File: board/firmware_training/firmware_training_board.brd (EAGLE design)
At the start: 68.6 x 53.4 mm, 17 parts, among them J1 GY-521-MPU-6050, SW1 PTS645, SW2 PTS645

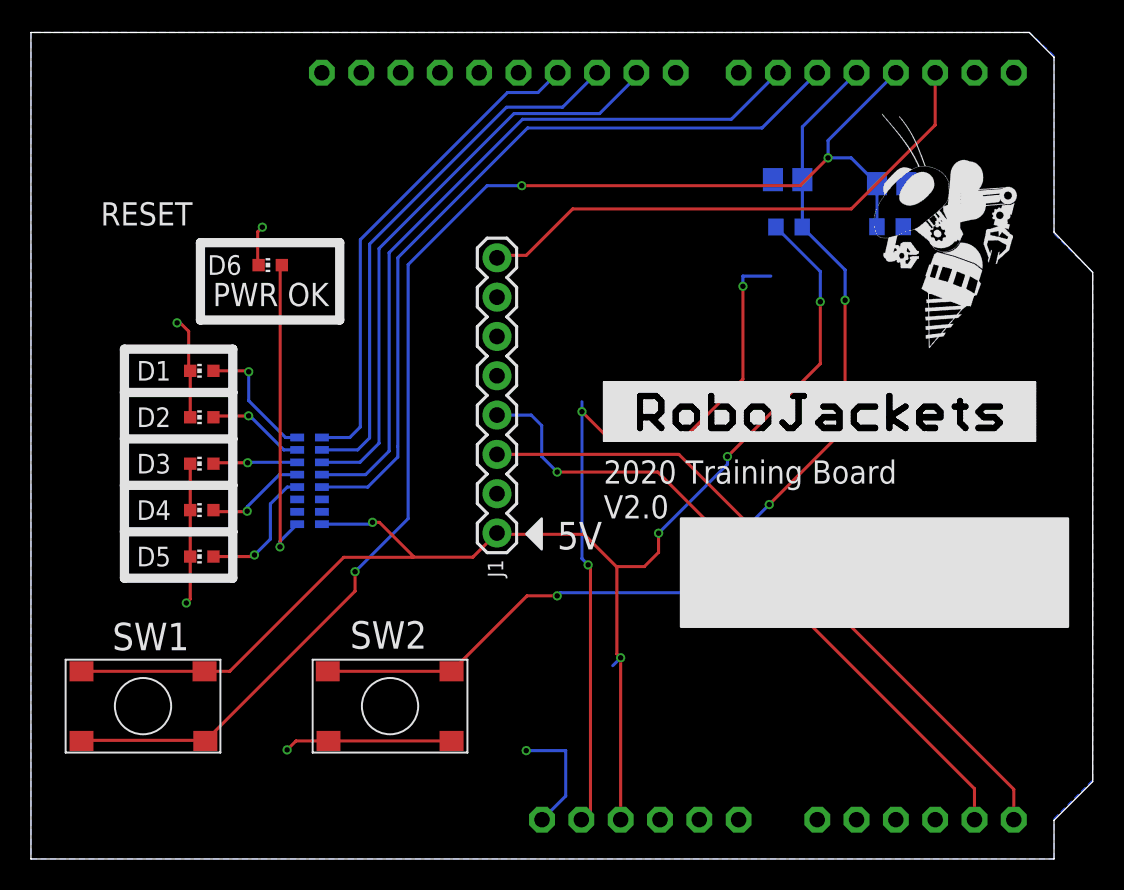
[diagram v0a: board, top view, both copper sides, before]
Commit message: Finished schematic, started board
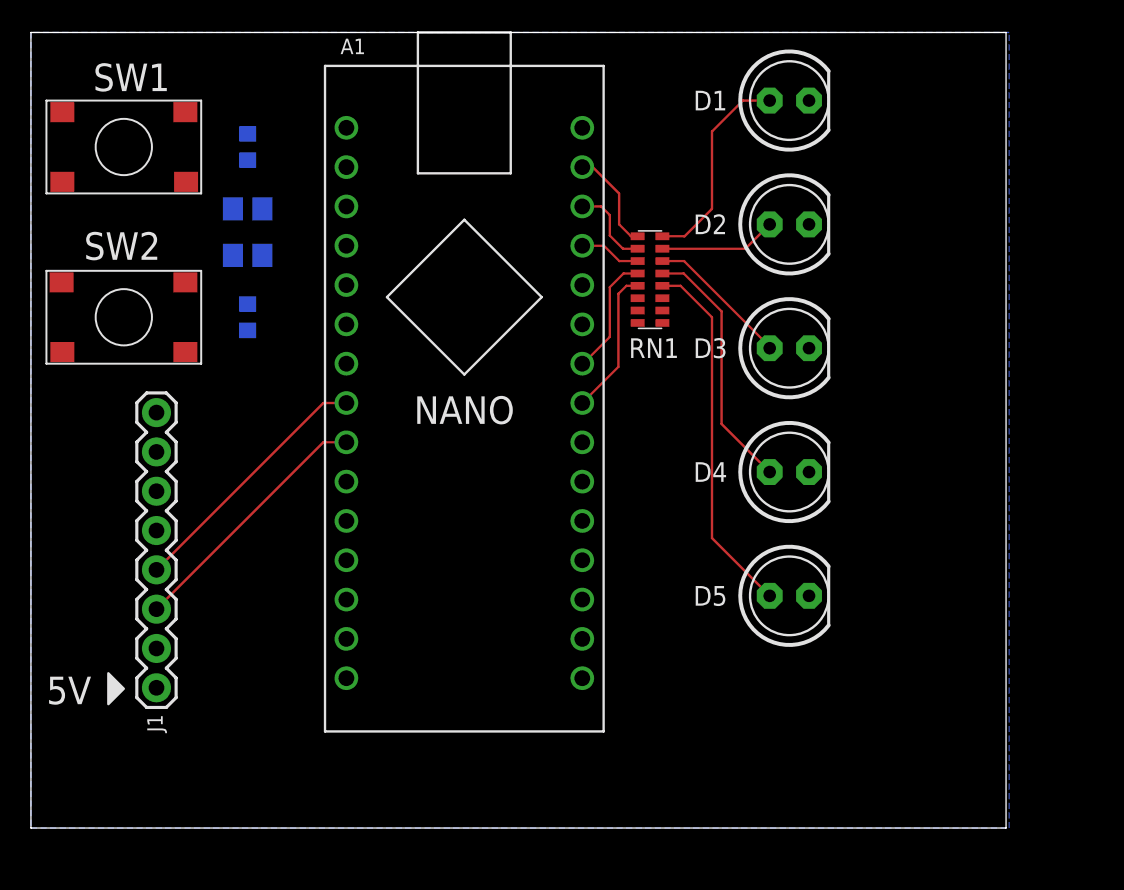
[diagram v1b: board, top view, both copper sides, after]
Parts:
- removed D6: GRN, led:CHIP-LED0603
- A1: value ARDUINOR3-NOIOREF-NOTEXT -> NANO; device adafruit:ARDUINOR3-NOTEXT-NOIOREF -> firmware_training_board:NANO
- D1: device led:CHIP-LED0603 -> adafruit:LED5MM
- D2, D3, D4, D5: device led:CHIP-LED0603 -> firmware_training_board:LED5MM
- moved R8 41.8 mm to (14.0, 46.0), turned to 90 degrees
- moved D1 41.8 mm to (49.0, 49.0), turned to 0 degrees
- moved C1 41.6 mm to (14.0, 42.0)
- moved A1 41.0 mm to (28.0, 30.0)
- moved D2 40.0 mm to (49.0, 41.0), turned to 0 degrees
- moved D3 38.7 mm to (49.0, 33.0), turned to 0 degrees
- moved D5 38.0 mm to (49.0, 17.0), turned to 0 degrees
- moved D4 38.0 mm to (49.0, 25.0), turned to 0 degrees
- moved SW1 36.1 mm to (6.00, 46.0)
- moved R10 35.5 mm to (14.0, 35.0), turned to 270 degrees
- moved C2 35.2 mm to (14.0, 39.0), turned to 180 degrees
- moved U$4 33.4 mm to (37.0, 7.00), flipped to the bottom, turned to 90 degrees
- moved SW2 30.4 mm to (6.00, 35.0)
- moved RN1 25.6 mm to (40.0, 37.4), flipped to the top
- moved J1 24.2 mm to (8.11, 11.1)
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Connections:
- net N$2 renamed D1_LED
- net N$3 renamed D2_LED
- net N$4 renamed D3_LED
- net N$5 renamed D4_LED
- net N$6 renamed D5_LED
- removed net N$9: D6.A, RN1.9
- removed net VIN: A1.VIN
- net !RESET: now also A1.RST; no longer A1.RESET
- net +3.3V: now also A1.3.3V; no longer A1.3V
- net +5V: no longer RN1.8
- net GND: now also D1.K, D2.K, D3.K, D4.K, D5.K; no longer A1.GND2, D1.C, D2.C, D3.C, D4.C, D5.C, D6.C
- net MPU_INT: now also A1.D3; no longer A1.D2
- net SW1_INT: now also A1.D2; no longer A1.D3
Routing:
- net +5V: track 93.0 -> 0.00 mm, vias 5 -> 0
- net SW1_INT: track 88.3 -> 0.00 mm, vias 3 -> 0
- net !SW2_INPUT: track 65.5 -> 0.00 mm, vias 3 -> 0
- net +3.3V: track 48.5 -> 0.00 mm, vias 3 -> 0
- net D5_CTRL: track 50.6 -> 9.48 mm
- net D4_CTRL: track 47.7 -> 7.88 mm
- net MPU_INT: track 35.2 -> 0.00 mm
- net D3_CTRL: track 38.3 -> 3.99 mm
- net D2_CTRL: track 35.2 -> 5.48 mm
- net GND: track 29.1 -> 0.00 mm, vias 4 -> 0
- net SCL: track 44.3 -> 16.7 mm
- net SDA: track 44.0 -> 16.7 mm, vias 1 -> 0
- net D1_CTRL: track 32.1 -> 6.60 mm
- net N$9: track 20.2 -> 0.00 mm, vias 1 -> 0
- net D5_LED: track 8.60 -> 23.6 mm, vias 1 -> 0
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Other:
- board size 68.6 x 53.4 mm -> 63 x 51.4 mm
- board text removed: "PWR OK"
- board text removed: "RESET"
